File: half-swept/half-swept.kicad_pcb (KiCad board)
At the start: 2 copper layers, 109.4 x 87.5 mm, 26 parts, among them J2 AudioJack4dpb, SW1 SW_Push, SW10 SW_Push, SW11 SW_Push, SW12 SW_Push, SW13 SW_Push, SW14 SW_Push, SW15 SW_Push, SW16 SW_Push, SW17 SW_Push, SW2 SW_Push, SW3 SW_Push, SW4 SW_Push, SW5 SW_Push, SW6 SW_Push, SW7 SW_Push, SW8 SW_Push, SW9 SW_Push, U1 ProMicro-kbd

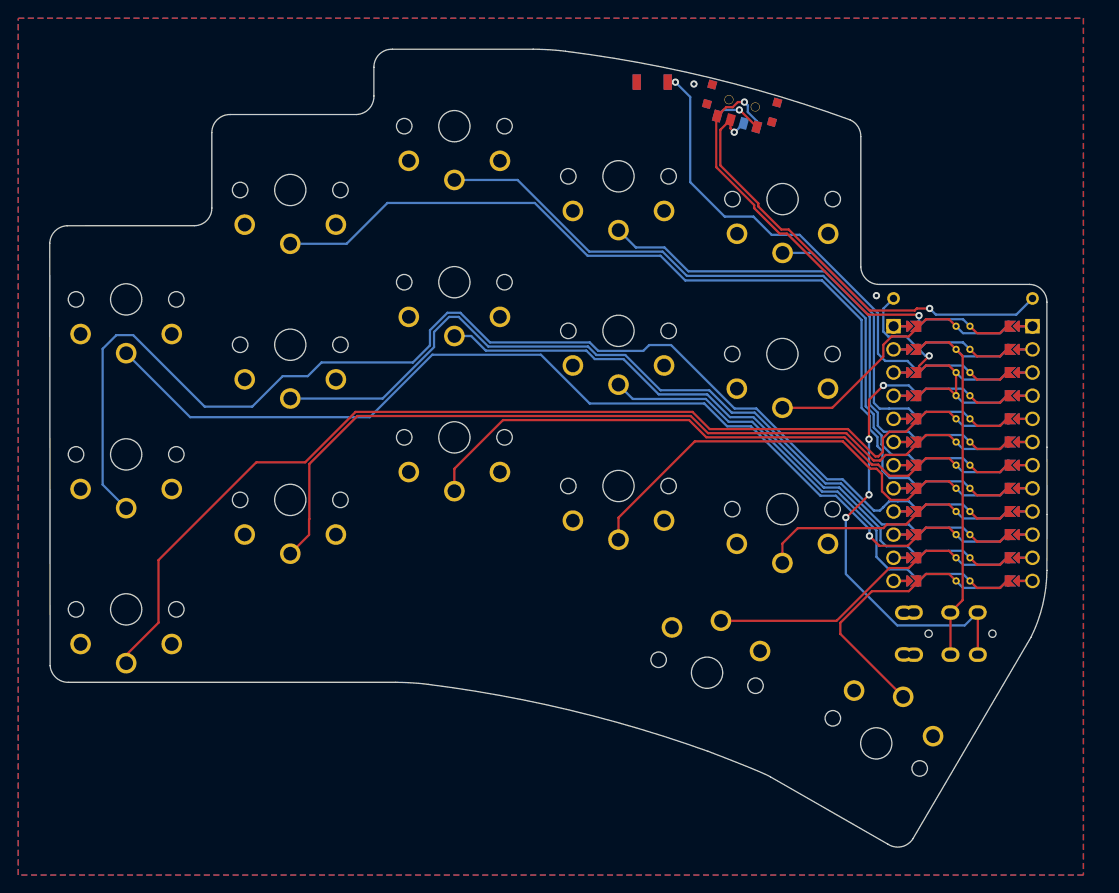
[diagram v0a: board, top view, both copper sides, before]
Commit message: final -- add cool silkscreen, reduce errors and wardnings from kicad
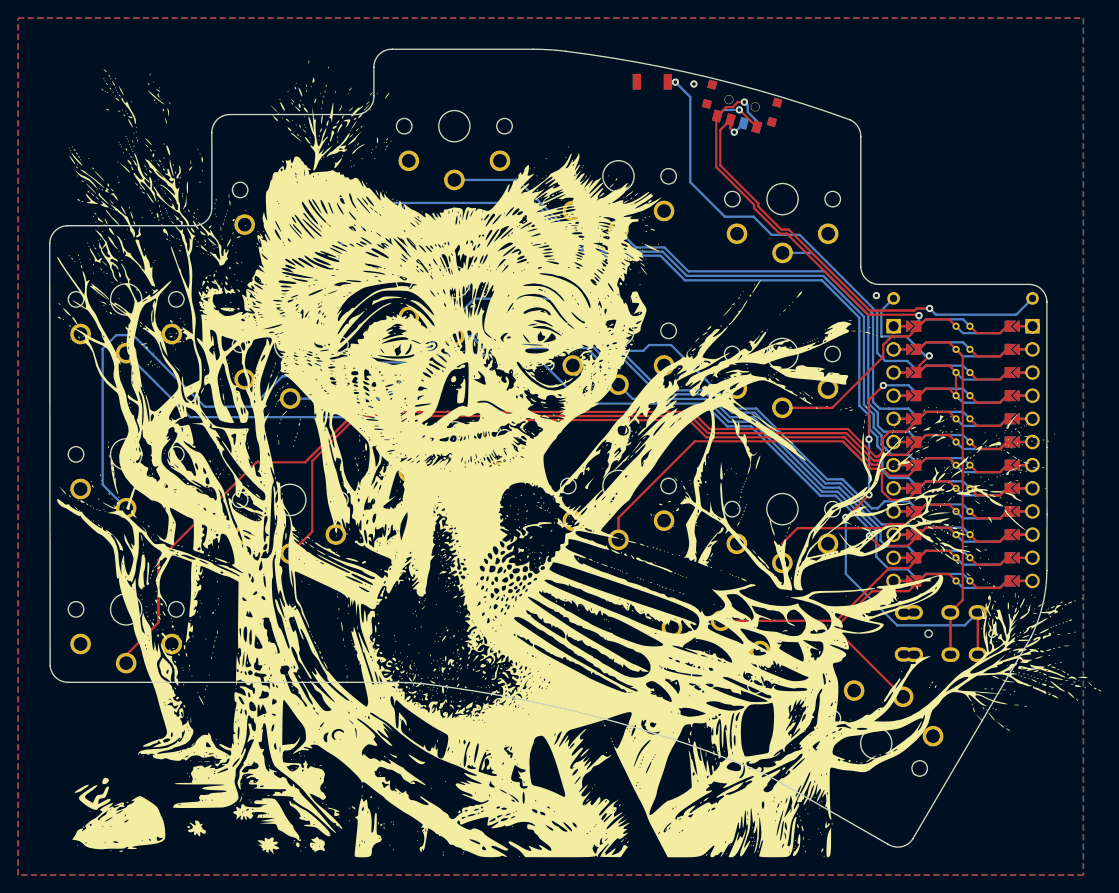
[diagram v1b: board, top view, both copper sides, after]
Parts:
- removed the G*** at (71.5, 78.0)
- removed the G*** at (54.0, 84.5)
- added G***: LOGO, half-swept:owl, F.Cu at (83.0, 62.0)
- added G***: LOGO, LOGO, B.Cu at (51.0, 82.0)
- added G***: LOGO, LOGO, B.Cu at (70.5, 85.5)
- moved RSW2 0.05 mm to (84.8, 22.2)
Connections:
- RSW2 pad 1: gnd -> (no net)
- RSW2 pad 2: gnd -> (no net)
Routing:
- net Switch6: track 127.6 -> 128.7 mm
- net reset: track 49.7 -> 48.8 mm
- net gnd: track 15.1 -> 15.7 mm
